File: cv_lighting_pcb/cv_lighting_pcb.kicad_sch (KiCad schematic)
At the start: 10 parts

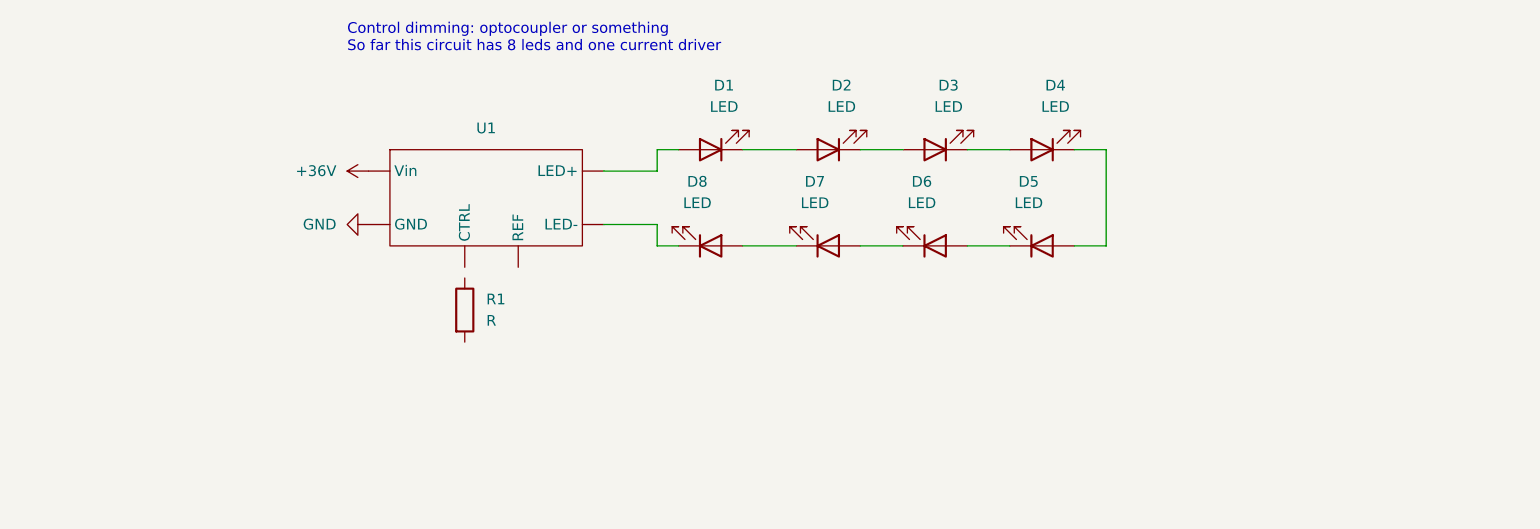
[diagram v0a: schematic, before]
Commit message: cv lighting schematic
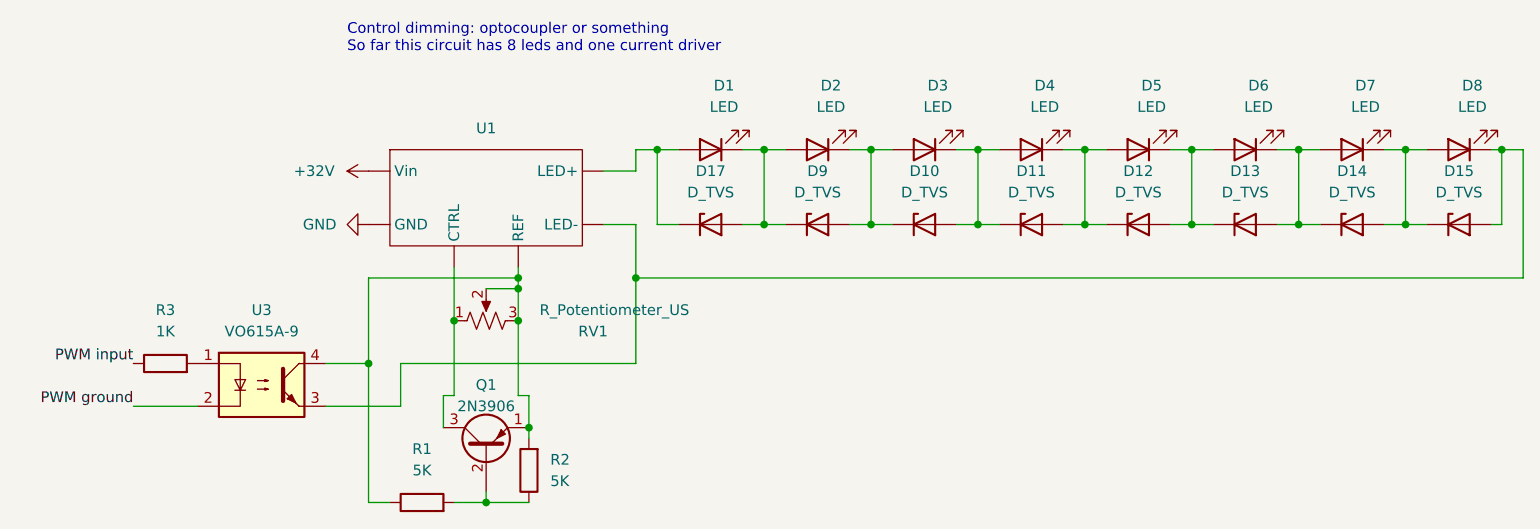
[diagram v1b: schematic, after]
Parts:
- added +32V: ~, symbol cv_lighting_symbols:+32V
- added D10, D11, D12, D13, D14, D15, D17, D9: D_TVS, symbol Device:D_Zener
- added Q1: 2N3906, Package_TO_SOT_THT:TO-92_Inline, symbol Transistor_BJT:2N3906
- added R2: 5K, symbol Device:R
- added R3: 1K, symbol Device:R
- added RV1: R_Potentiometer_US, symbol Device:R_Potentiometer_US
- added U3: VO615A-9, symbol Isolator:VO615A-9
- R1: value R -> 5K
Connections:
- net +36V is gone; now on net GND: U1. (Vin)
- net at D1.1 (K), D2.2 (A): now also D17.2 (A), D9.1 (K)
- net at D1.2 (A), U1. (Vin): now also D17.1 (K)
- net at D4.1 (K), D5.2 (A): now also D11.2 (A), D12.1 (K)
- net at D3.1 (K), D4.2 (A): now also D10.2 (A), D11.1 (K)
- net at D8.1 (K), U1. (Vin): now also D15.2 (A), U3.3
- net at D5.1 (K), D6.2 (A): now also D12.2 (A), D13.1 (K)
- net at D2.1 (K), D3.2 (A): now also D10.1 (K), D9.2 (A)
- net at D7.1 (K), D8.2 (A): now also D14.2 (A), D15.1 (K)
- net at D6.1 (K), D7.2 (A): now also D13.2 (A), D14.1 (K)
- net at R1.1: now also U1. (Vin), Q1.1 (E), R2.2, RV1.2, RV1.3, U3.4
- net at R1.2: now also Q1.2 (B), R2.1
- new net: Q1.3 (C), RV1.1, U1. (Vin)
- new net: R3.2, U3.1
- new net +32V: +32V.1 (+32V), U1. (Vin)
- new net PWM ground: U3.2
- new net PWM input: R3.1
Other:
- moved on the sheet: D2, D3, D4, D5, D6, D7, D8
